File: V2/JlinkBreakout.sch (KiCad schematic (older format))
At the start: 11 parts, among them J1 JLINK, J2 TC, J3 SWD, U1 SGM2019, U2 switch_0204

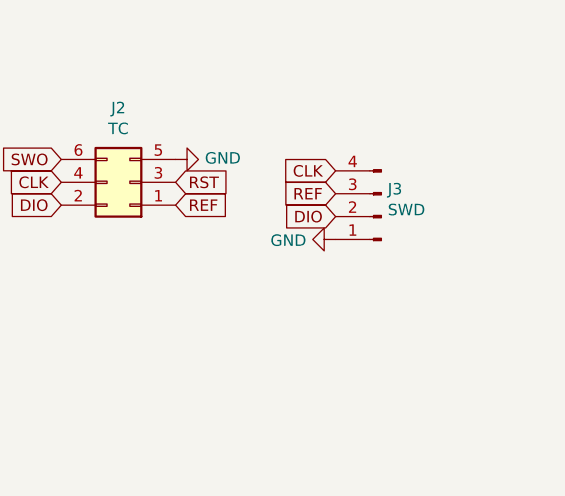
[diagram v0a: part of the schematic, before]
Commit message: finalized V2
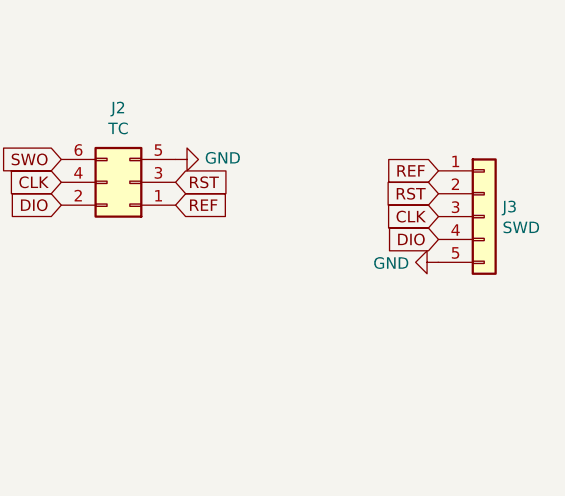
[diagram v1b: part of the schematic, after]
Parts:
- removed J3: SWD, Connector_JST:JST_XH_B4B-XH-A_1x04_P2.50mm_Vertical, symbol Connector:Conn_01x04_Male
- added J3: SWD, Connector_JST:JST_XH_B5B-XH-A_1x05_P2.50mm_Vertical, symbol Connector_Generic:Conn_01x05
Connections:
- net CLK: now also J3.3 (Pin_3)
- net DIO: now also J3.4 (Pin_4)
- net GND: now also J3.5 (Pin_5)
- net REF: now also J3.1 (Pin_1)
- net RST: now also J3.2 (Pin_2)
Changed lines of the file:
@@
 L power:GND #PWR0106
 U 1 1 5CD07720
-P 7850 4300
-F 0 "#PWR0106" H 7850 4050 50  0001 C CNN
-F 1 "GND" V 7855 4172 50  0000 R CNN
-F 2 "" H 7850 4300 50  0001 C CNN
-F 3 "" H 7850 4300 50  0001 C CNN
-	1    7850 4300
+P 8300 4400
+F 0 "#PWR0106" H 8300 4150 50  0001 C CNN
+F 1 "GND" V 8305 4272 50  0000 R CNN
+F 2 "" H 8300 4400 50  0001 C CNN
+F 3 "" H 8300 4400 50  0001 C CNN
+	1    8300 4400
 	0    1    1    0
 $EndComp
@@
 Text GLabel 5800 4300 2    50   Input ~ 0
 RST
-Text GLabel 7850 4000 0    50   Input ~ 0
+Text GLabel 8300 4200 0    50   Input ~ 0
 CLK
 Text GLabel 6650 4050 0    50   Input ~ 0
@@
 Text GLabel 5800 4000 2    50   Input ~ 0
 CLK
-Text GLabel 7850 4100 0    50   Input ~ 0
+Text GLabel 8300 4000 0    50   Input ~ 0
 REF
 Text GLabel 5800 3900 2    50   Input ~ 0
 DIO
-Text GLabel 7850 4200 0    50   Input ~ 0
+Text GLabel 8300 4300 0    50   Input ~ 0
 DIO
 Text GLabel 6650 4150 0    50   Input ~ 0
@@
 $EndComp
 $Comp
-L Connector:Conn_01x04_Male J3
-U 1 1 5DBC477C
-P 8050 4200
-F 0 "J3" H 8022 4080 50  0000 R CNN
-F 1 "SWD" H 8022 4171 50  0000 R CNN
-F 2 "Connector_JST:JST_XH_B4B-XH-A_1x04_P2.50mm_Vertical" H 8050 4200 50  0001 C CNN
-F 3 "~" H 8050 4200 50  0001 C CNN
-	1    8050 4200
-	-1   0    0    1
-$EndComp
-$Comp
 L otter:SGM2019 U1
 U 1 1 5DBCEBD6
@@
 	0    1    1    0
 $EndComp
+$Comp
+L Connector_Generic:Conn_01x05 J3
+U 1 1 5DBDC6F2
+P 8500 4200
+F 0 "J3" H 8580 4242 50  0000 L CNN
+F 1 "SWD" H 8580 4151 50  0000 L CNN
+F 2 "Connector_JST:JST_XH_B5B-XH-A_1x05_P2.50mm_Vertical" H 8500 4200 50  0001 C CNN
+F 3 "~" H 8500 4200 50  0001 C CNN
+	1    8500 4200
+	1    0    0    -1
+$EndComp
+Text GLabel 8300 4100 0    50   Input ~ 0
+RST
 $EndSCHEMATC
